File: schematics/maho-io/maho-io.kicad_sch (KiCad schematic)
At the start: 60 parts, among them J1 PWR, J2 V2, J3 V1

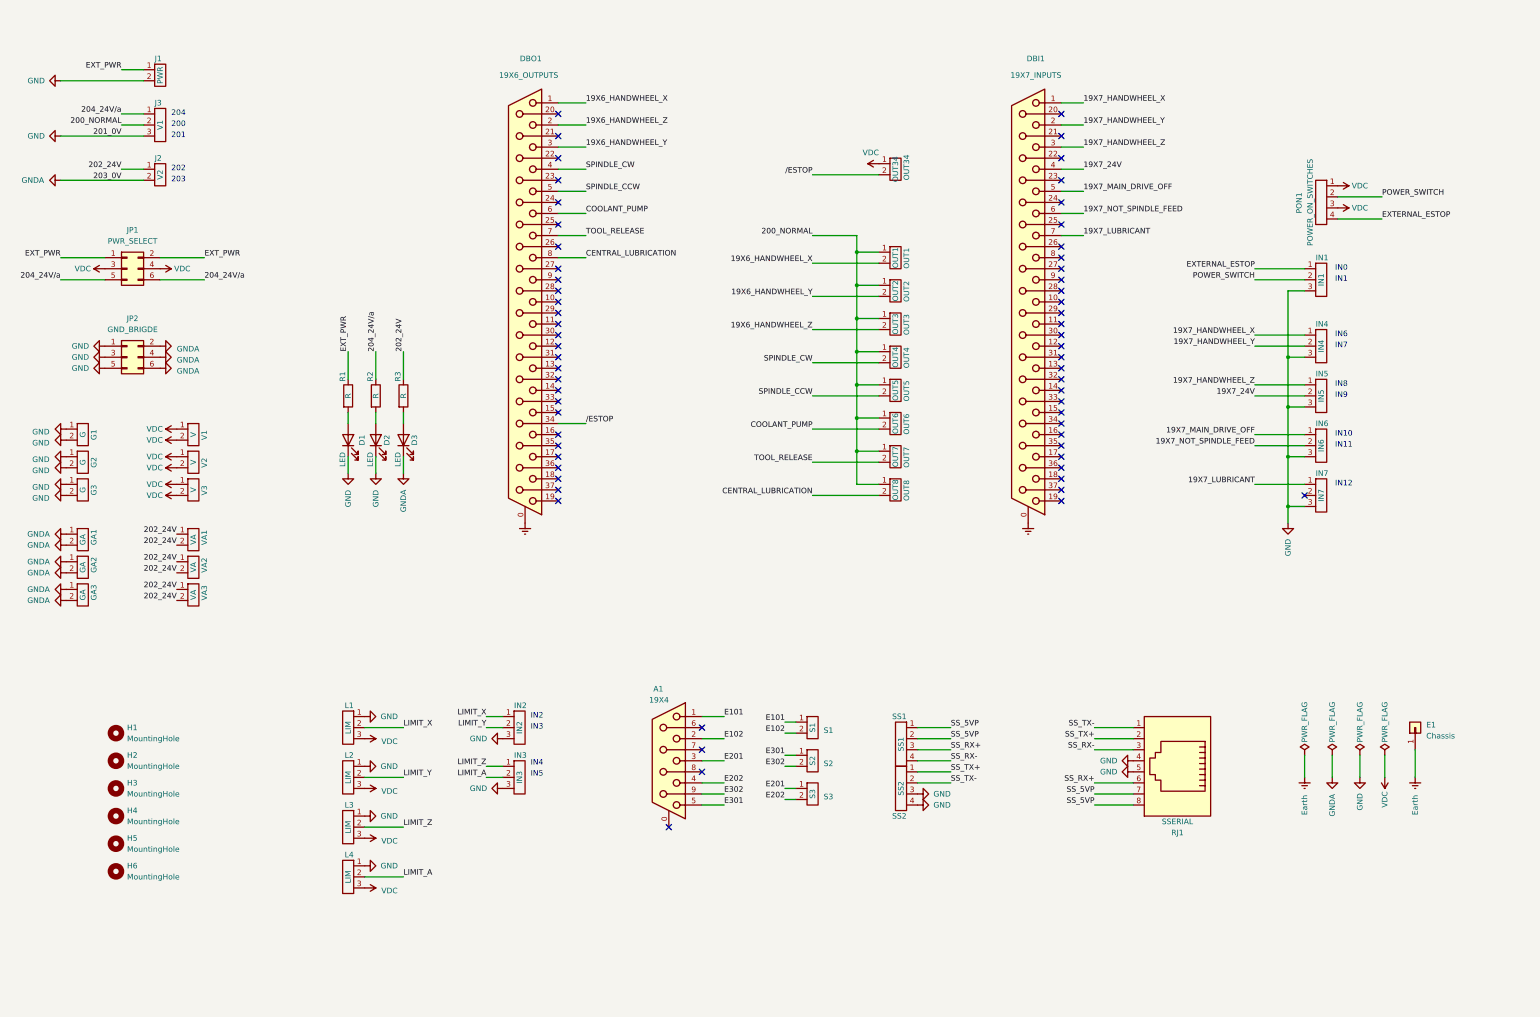
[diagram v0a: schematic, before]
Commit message: board
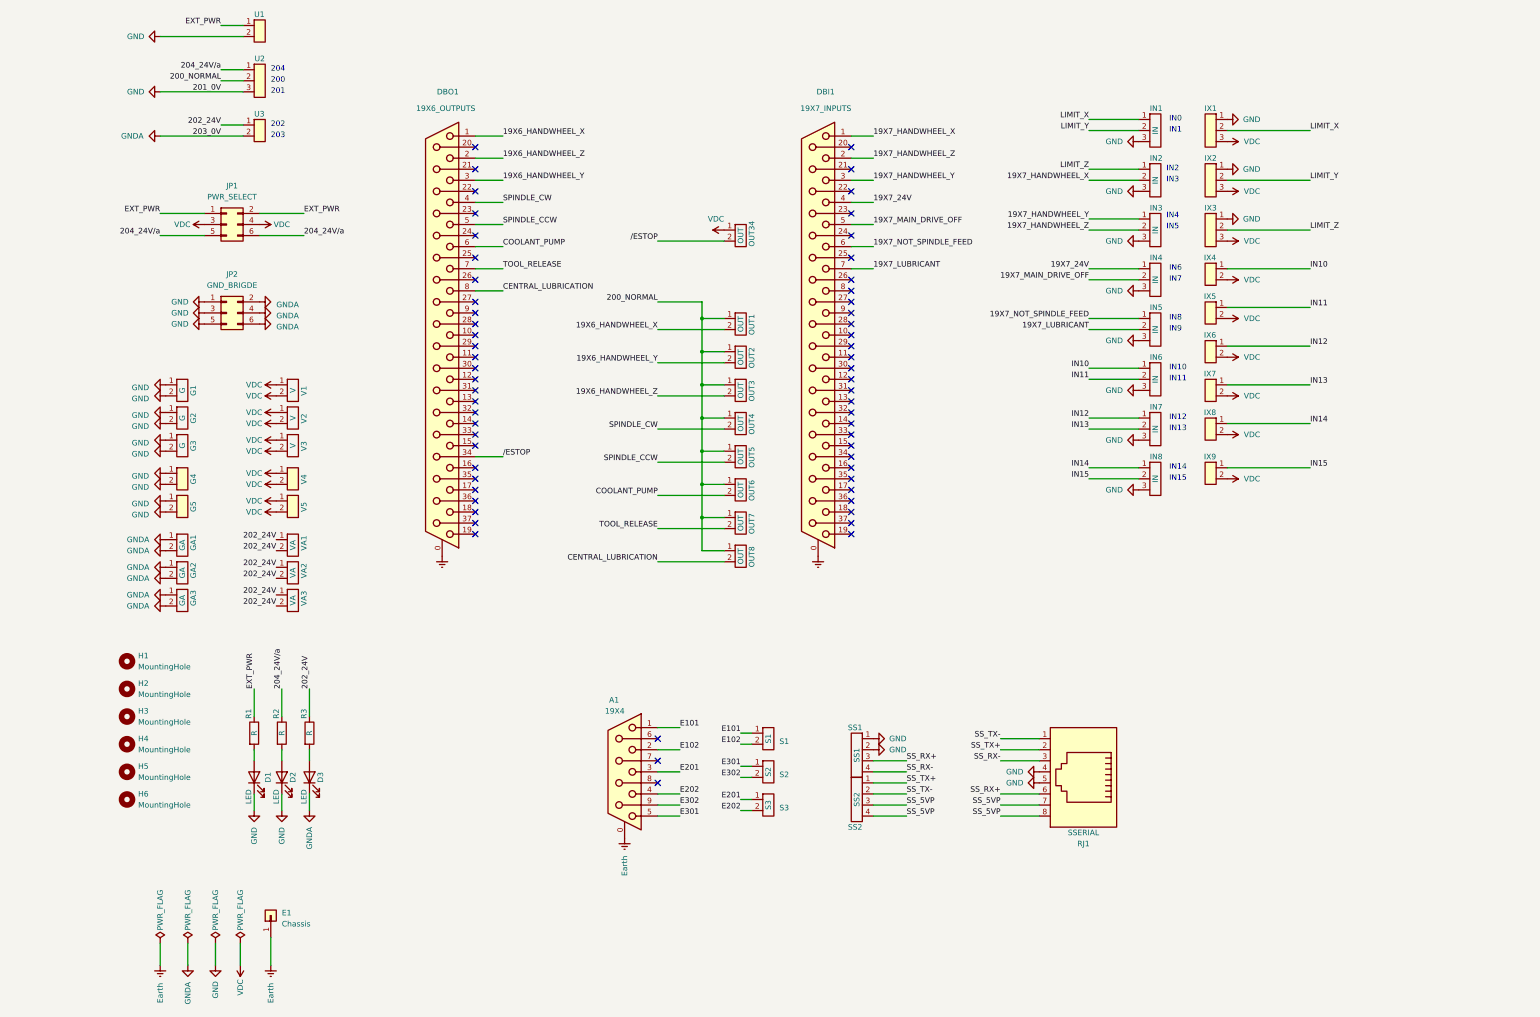
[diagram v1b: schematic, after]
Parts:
- removed J1: PWR, XY2500V-C(5.08)-2P:XY2500V-C(5.08)-2P, symbol XY2500V-C(5.08)-2P:XY2500V-C(5.08)-2P
- removed J2: V2, XY2500V-C(5.08)-2P:XY2500V-C(5.08)-2P, symbol XY2500V-C(5.08)-2P:XY2500V-C(5.08)-2P
- removed J3: V1, XY2500V-C(5.08)-3P:XY2500V-C(5.08)-3P, symbol XY2500V-C(5.08)-3P:XY2500V-C(5.08)-3P
- removed L1, L2, L3, L4: LIM, XY2500V-C(5.08)-3P:XY2500V-C(5.08)-3P, symbol XY2500V-C(5.08)-3P:XY2500V-C(5.08)-3P
- removed PON1: POWER_ON_SWITCHES, XY2500V-C(5.08)-4P:XY2500V-C(5.08)-4P, symbol XY2500V-C(5.08)-4P:XY2500V-C(5.08)-4P
- added G4, G5, IX4, IX5, IX6, IX7, IX8, IX9, U1, U3, V4, V5: XY2500R-C(5.08)-2P, XY2500R-C(5.08)-2P:XY2500R-C(5.08)-2P, symbol XY2500R-C(5.08)-2P:XY2500R-C(5.08)-2P
- added IN8: IN, XY2500V-C(5.08)-3P:XY2500V-C(5.08)-3P, symbol XY2500V-C(5.08)-3P:XY2500V-C(5.08)-3P
- added IX1, IX2, IX3, U2: XY2500R-C(5.08)-3P, XY2500R-C(5.08)-3P:XY2500R-C(5.08)-3P, symbol XY2500R-C(5.08)-3P:XY2500R-C(5.08)-3P
- IN1: value IN1 -> IN
- IN2: value IN2 -> IN
- IN3: value IN3 -> IN
- IN4: value IN4 -> IN
- IN5: value IN5 -> IN
- IN6: value IN6 -> IN
- IN7: value IN7 -> IN
- OUT1: value OUT1 -> OUT
- OUT2: value OUT2 -> OUT
- OUT3: value OUT3 -> OUT
- OUT34: value OUT34 -> OUT
- OUT4: value OUT4 -> OUT
- OUT5: value OUT5 -> OUT
- OUT6: value OUT6 -> OUT
- OUT7: value OUT7 -> OUT
- OUT8: value OUT8 -> OUT
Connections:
- net EXTERNAL_ESTOP is gone; now on net LIMIT_X: IN1.1
- net LIMIT_Α is gone; now on net 19X7_HANDWHEEL_Z: IN3.2
- net POWER_SWITCH is gone; now on net LIMIT_Υ: IN1.2
- net 19X7_24V: now also IN4.1; no longer IN5.2
- net 19X7_HANDWHEEL_X: now also IN2.2; no longer IN4.1
- net 19X7_HANDWHEEL_Y: now also DBI1.3, IN3.1; no longer DBI1.2, IN4.2
- net 19X7_HANDWHEEL_Z: now also DBI1.2; no longer DBI1.3, IN5.1
- net 19X7_LUBRICANT: now also IN5.2; no longer IN7.1
- net 19X7_MAIN_DRIVE_OFF: now also IN4.2; no longer IN6.1
- net 19X7_NOT_SPINDLE_FEED: now also IN5.1; no longer IN6.2
- net 200_NORMAL: now also U2.2
- net 202_24V: now also U3.1
- net 204_24V/a: now also U2.1
- net EXT_PWR: now also U1.1
- net Earth: now also A1.0 (PAD)
- net GND: now also SS1.1, SS1.2, G4.1, G4.2, G5.1, G5.2, IN8.3, IX1.1, IX2.1, IX3.1, U1.2, U2.3; no longer SS2.3, SS2.4
- net GNDA: now also U3.2
- net LIMIT_X: now also IX1.2; no longer IN2.1
- net LIMIT_Ζ: now also IN2.1, IX3.2; no longer IN3.1
- net LIMIT_Υ: now also IX2.2; no longer IN2.2
- net SS_5VP: now also SS2.3, SS2.4; no longer SS1.1, SS1.2
- net VDC: now also IX1.3, IX2.3, IX3.3, IX4.2, IX5.2, IX6.2, IX7.2, IX8.2, IX9.2, V4.1, V4.2, V5.1, V5.2
- net IN13: now reaches IN7.2
- net IN13: now also IX7.1
- new net IN10: IN6.1, IX4.1
- new net IN11: IN6.2, IX5.1
- new net IN12: IN7.1, IX6.1
- new net IN14: IN8.1, IX8.1
- new net IN15: IN8.2, IX9.1
- no-connect marks 63 -> 61
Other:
- note added: "IN13"
- note added: "IN14"
- note added: "IN15"
- moved on the sheet: A1, D1, D2, D3, DBI1, DBO1, E1, G1, G2, G3, GA1, GA2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

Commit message: maho-io release for fab
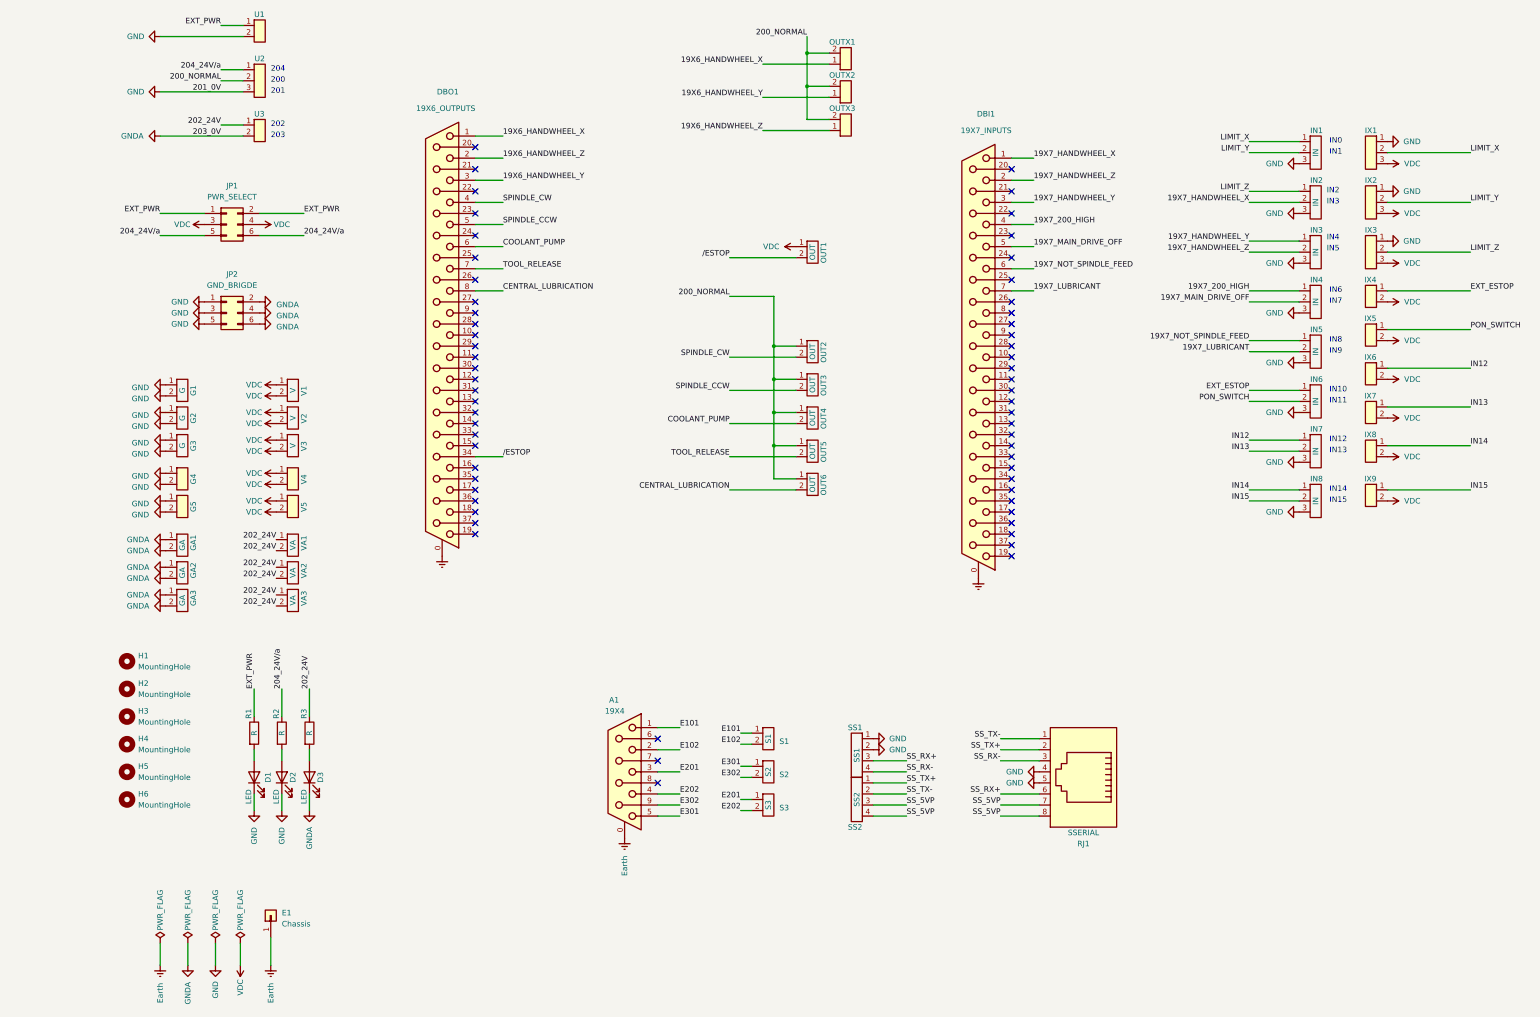
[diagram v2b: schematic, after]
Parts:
- removed OUT1, OUT2, OUT3: OUT, XY2500V-C(5.08)-2P:XY2500V-C(5.08)-2P, symbol XY2500V-C(5.08)-2P:XY2500V-C(5.08)-2P
- added OUTX1, OUTX2, OUTX3: XY2500R-C(5.08)-2P, XY2500R-C(5.08)-2P:XY2500R-C(5.08)-2P, symbol XY2500R-C(5.08)-2P:XY2500R-C(5.08)-2P
- renumbered OUT34 to OUT1, OUT4 to OUT2, OUT5 to OUT3, OUT6 to OUT4, OUT7 to OUT5, OUT8 to OUT6
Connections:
- net 19X6_HANDWHEEL_X: now also OUTX1.1
- net 19X6_HANDWHEEL_Y: now also OUTX2.1
- net 19X6_HANDWHEEL_Z: now also OUTX3.1
- net 200_NORMAL: now also OUTX1.2, OUTX2.2, OUTX3.2
- net 19X7_24V renamed 19X7_200_HIGH
- net IN10 renamed EXT_ESTOP
- net IN11 renamed PON_SWITCH
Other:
- moved on the sheet: DBI1, IN1, IN2, IN3, IN4, IN5, IN6, IN7, IN8, IX1, IX2, IX3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
